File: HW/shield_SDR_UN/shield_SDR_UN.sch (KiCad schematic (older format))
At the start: 0 parts

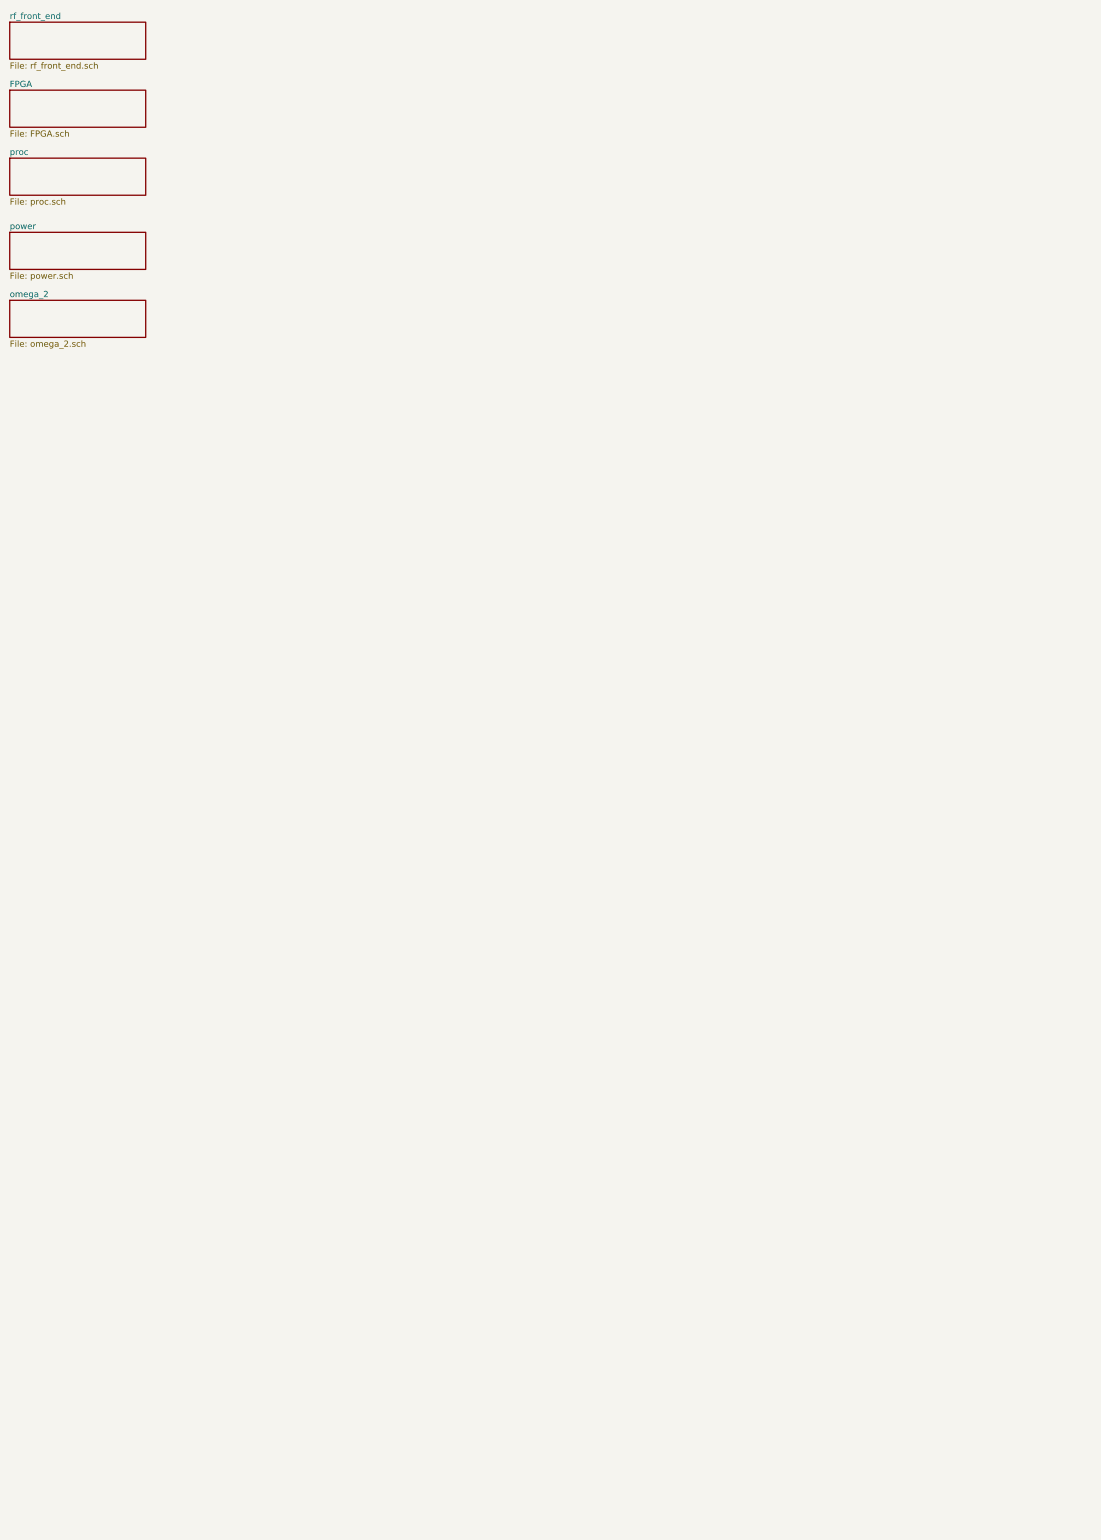
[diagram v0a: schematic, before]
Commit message: data bus proc-fpga
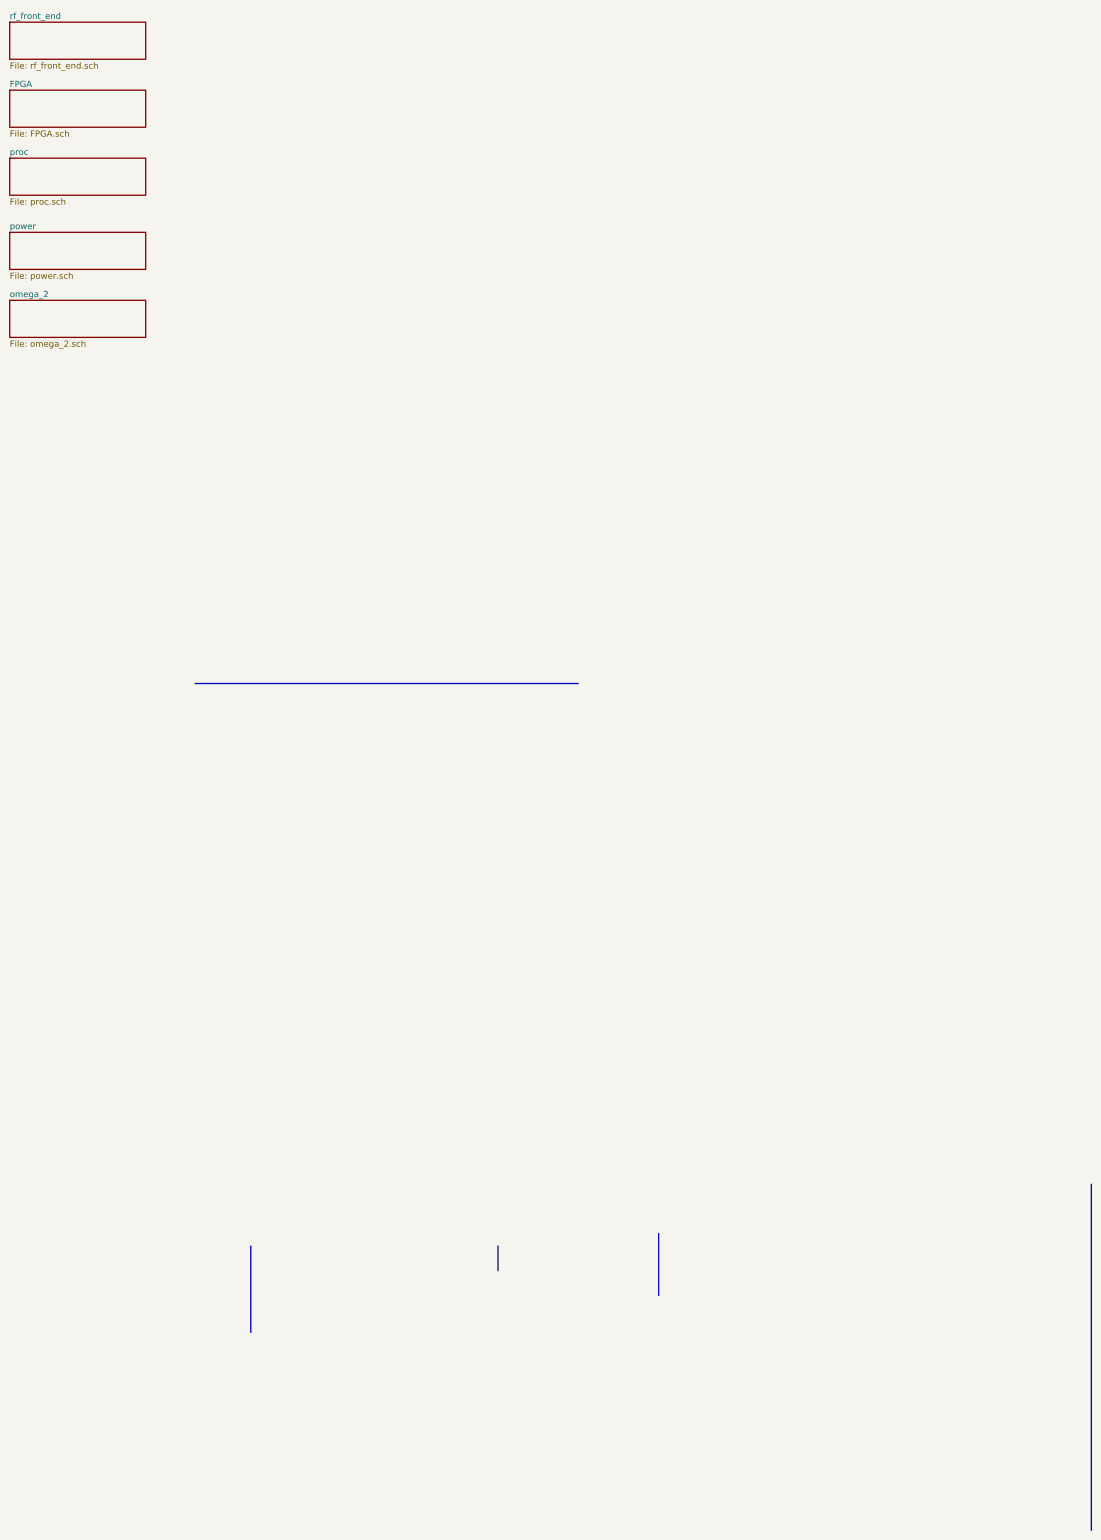
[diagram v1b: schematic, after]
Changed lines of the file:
@@
 F1 "omega_2.sch" 50
 $EndSheet
+Wire Bus Line
+	12650 12200 12650 15000
+Wire Bus Line
+	9150 12600 9150 13100
+Wire Bus Line
+	7850 12700 7850 12900
+Wire Bus Line
+	5850 12700 5850 13400
+Wire Bus Line
+	5400 8150 8500 8150
 $EndSCHEMATC

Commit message: algunos footprint_v2
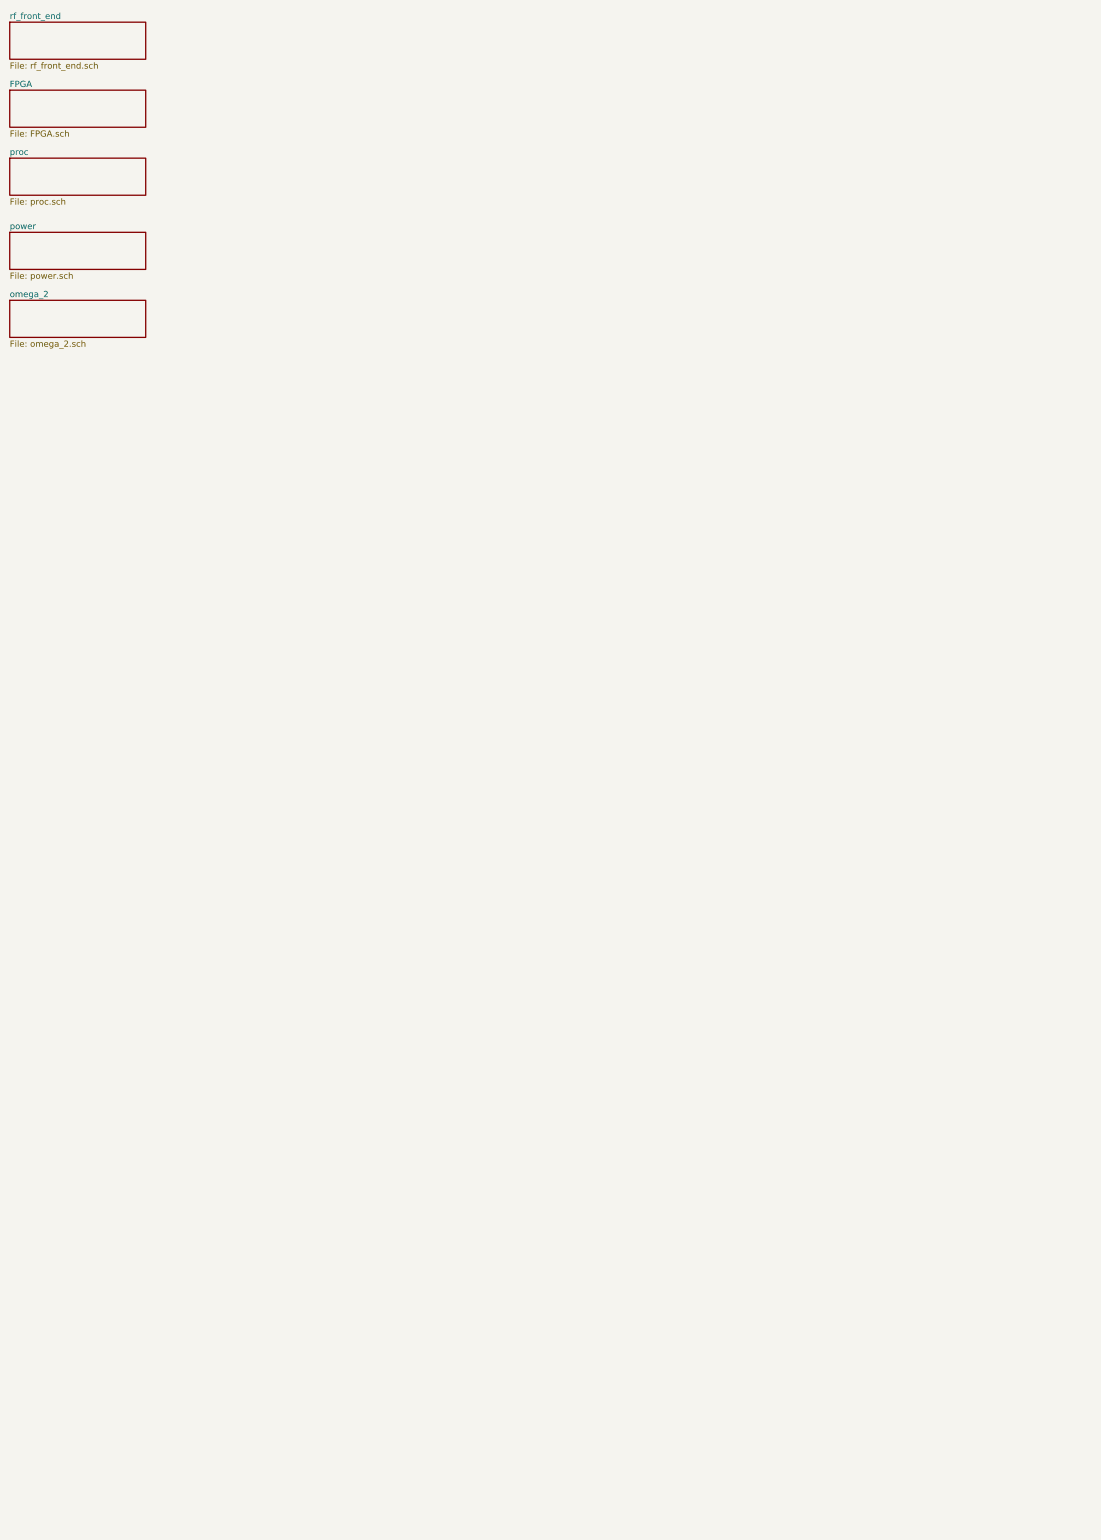
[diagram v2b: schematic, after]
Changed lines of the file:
@@
 F1 "omega_2.sch" 50
 $EndSheet
-Wire Bus Line
-	12650 12200 12650 15000
-Wire Bus Line
-	9150 12600 9150 13100
-Wire Bus Line
-	7850 12700 7850 12900
-Wire Bus Line
-	5850 12700 5850 13400
-Wire Bus Line
-	5400 8150 8500 8150
 $EndSCHEMATC
